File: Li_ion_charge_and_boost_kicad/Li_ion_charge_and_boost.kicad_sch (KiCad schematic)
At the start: 26 parts, among them J3 Boost_+, J4 Boost_-, U1 TP4056, U2 Type_C_6_pin, U3 DW01A, U5 MT3608

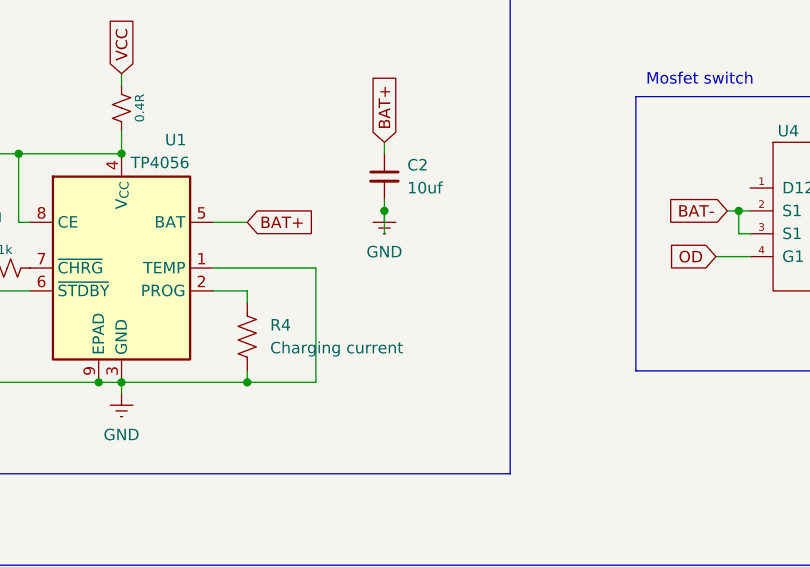
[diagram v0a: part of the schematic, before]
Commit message: Charging current and Inductor yet to confirm
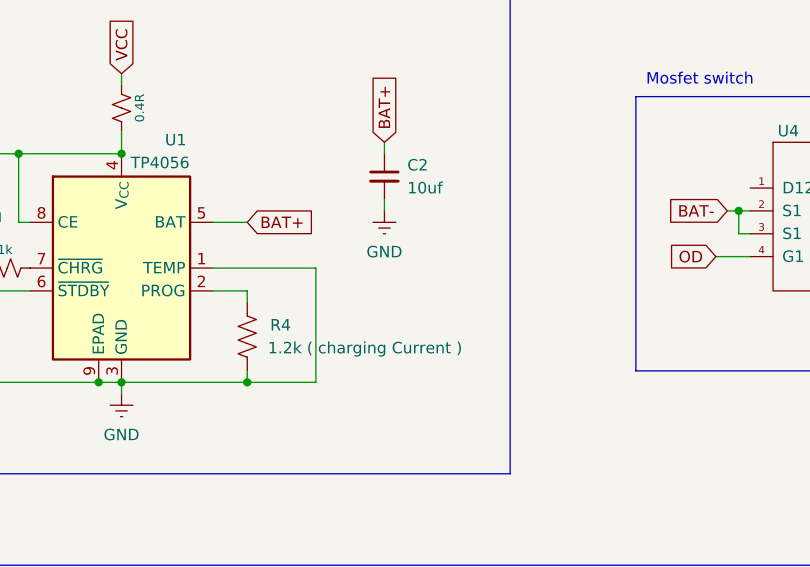
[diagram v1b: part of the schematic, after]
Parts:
- R4: value Charging current -> 1.2k ( charging Current )
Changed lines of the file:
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@@
 	)
 	(junction
-		(at 93.98 105.41)
-		(diameter 0)
-		(color 0 0 0 0)
-	)
-	(junction
 		(at 257.81 67.31)
 		(diameter 0)
@@
 	(wire
 		(pts
-			(xy 93.98 105.41) (xy 93.98 107.95)
-		)
-		(stroke
-			(width 0)
-			(type default)
-		)
-	)
-	(wire
-		(pts
 			(xy 93.98 97.79) (xy 93.98 99.06)
 		)
@@
 		(on_board yes)
 		(dnp no)
-		(fields_autoplaced yes)
 		(property "Reference" "R4"
 			(at 81.28 118.1099 0)
@@
 			)
 		)
-		(property "Value" "Charging current"
-			(at 81.28 120.6499 0)
+		(property "Value" "1.2k   ( charging Current )"
+			(at 81.026 120.65 0)
 			(effects
 				(font
